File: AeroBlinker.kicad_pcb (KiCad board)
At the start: 2 copper layers, 41.8 x 28 mm, 33 parts, among them J1 LED_GND, J2 LED_GND, J3 LED_GND, J4 BATTERY, J5 RECEIVER, J6 USB_C_Receptacle_USB2.0_16P, Q1 AO3400A, SW2 SW_Push, U1 STM32F042F6Px, U2 USBLC6-2SC6, U3 TPS62162DGR

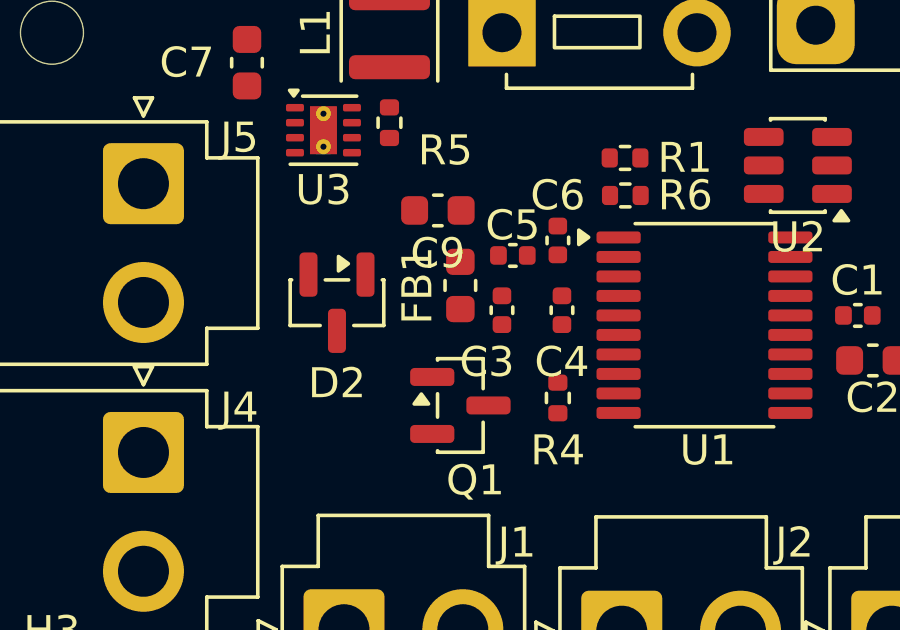
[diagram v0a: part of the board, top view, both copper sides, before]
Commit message: Autosave
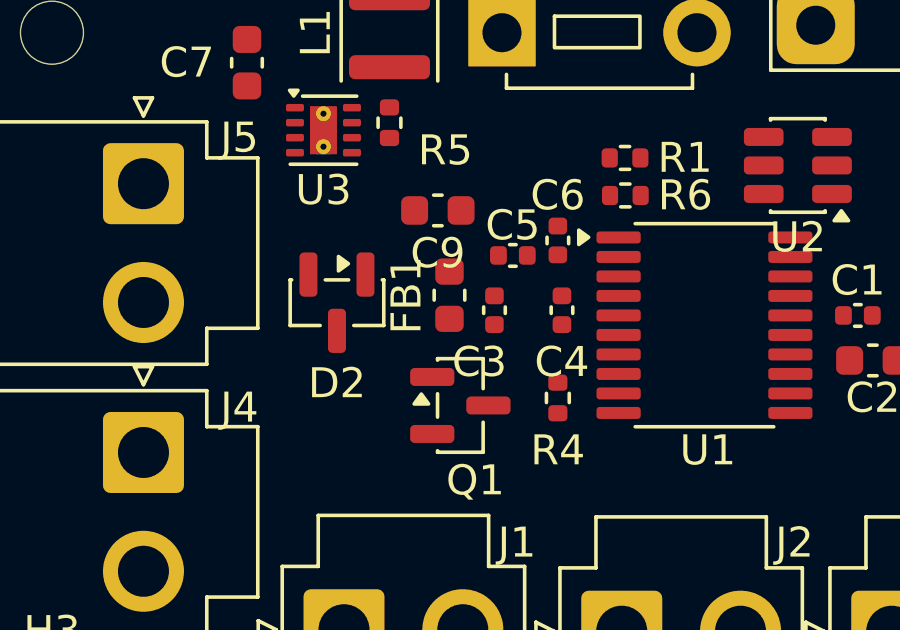
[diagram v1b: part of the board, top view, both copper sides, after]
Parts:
- moved FB1 0.49 mm to (140.5, 129.5)
- moved C3 0.25 mm to (142.0, 130.0)
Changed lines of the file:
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@@
 	(footprint "Capacitor_SMD:C_0402_1005Metric"
 		(layer "F.Cu")
-		(at 142.25 130 90)
+		(at 142 130 90)
 		(descr "Capacitor SMD 0402 (1005 Metric), square (rectangular) end terminal, IPC-7351 nominal, (Body size source: IPC-SM-782 page 76, https://www.pcb-3d.com/wordpress/wp-content/uploads/ipc-sm-782a_amendment_1_and_2.pdf)")
 		(tags "capacitor")
@@
 	(footprint "Inductor_SMD:L_0603_1608Metric"
 		(layer "F.Cu")
-		(at 140.8625 129.175 90)
+		(at 140.5 129.5 90)
 		(descr "Inductor SMD 0603 (1608 Metric), square (rectangular) end terminal, IPC-7351 nominal, (Body size source: http://www.tortai-tech.com/upload/download/2011102023233369053.pdf)")
 		(tags "inductor")
